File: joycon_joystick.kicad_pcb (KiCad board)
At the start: 2 copper layers, 35.1 x 23 mm, 2 parts, among them CN1 CONN_5POS, J1 Conn_01x05

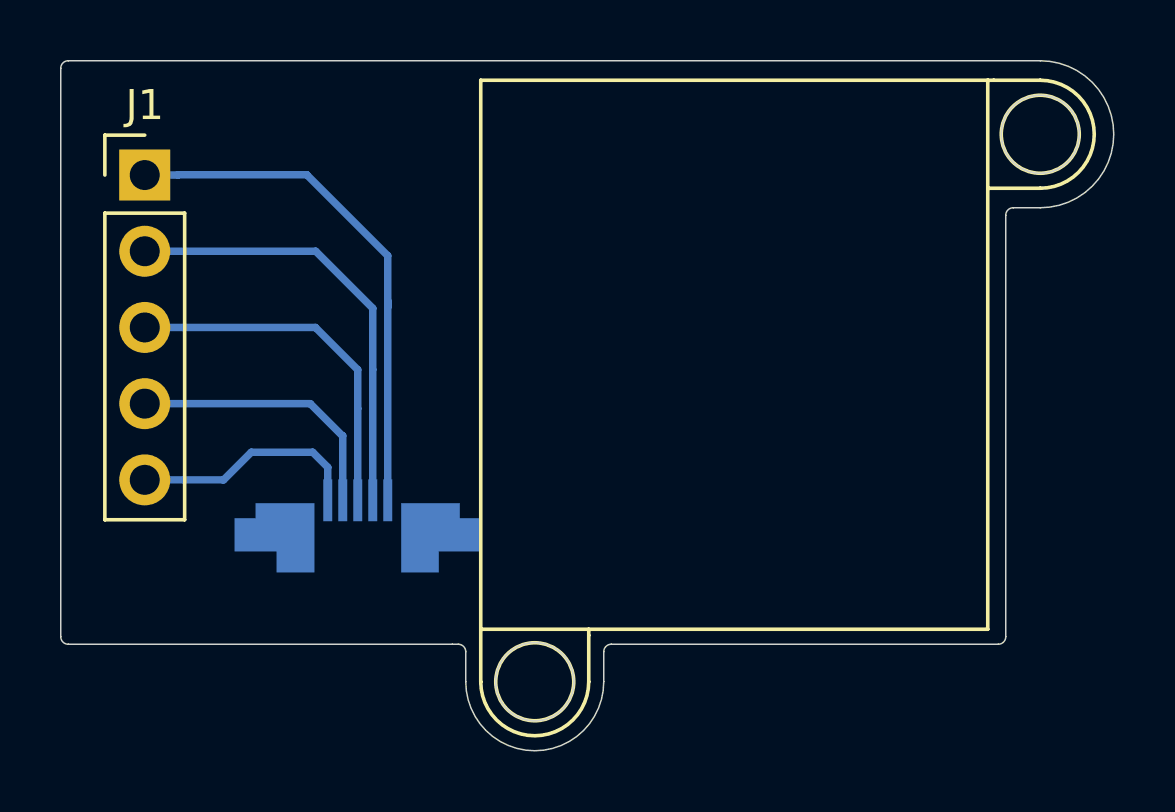
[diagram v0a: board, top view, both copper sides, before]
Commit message: took another shot at getting the geometry right
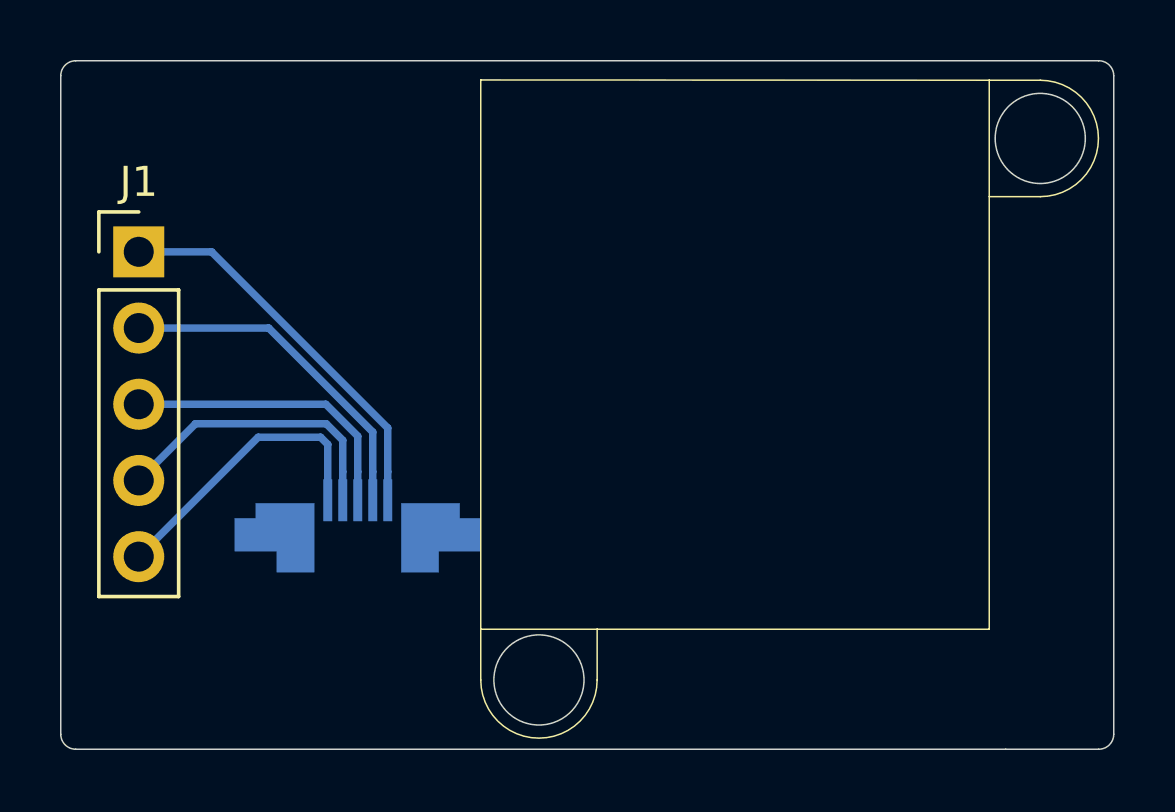
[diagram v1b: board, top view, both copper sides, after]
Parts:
- moved J1 2.57 mm to (117.6, 94.4)
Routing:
- net Net-(CN1-Pad1): track 17.6 -> 13.1 mm
- net Net-(CN1-Pad2): track 14.8 -> 11.5 mm
- net Net-(CN1-Pad3): track 12.0 -> 9.88 mm
- net Net-(CN1-Pad5): track 7.79 -> 9.91 mm
- net Net-(CN1-Pad4): track 9.19 -> 9.81 mm
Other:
- outline, holes or cut-outs redrawn
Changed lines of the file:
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@@
   (general
     (thickness 1.6)
-    (drawings 41)
-    (tracks 24)
+    (drawings 29)
+    (tracks 21)
     (zones 0)
     (modules 2)
@@
   )
   (module Connector_PinHeader_2.54mm:PinHeader_1x05_P2.54mm_Vertical (layer F.Cu)
-    (at 117.8 91.86)
+    (at 117.6 94.42)
     (descr "Through hole straight pin header, 1x05, 2.54mm pitch, single row")
     (tags "Through hole pin header THT 1x05 2.54mm single row")
@@
     )
   )
-  (gr_circle (center 130.8 108.75) (end 129.7 109.45) (layer Edge.Cuts) (width 0.05))
-  (gr_circle (center 147.65 90.5) (end 148.95 90.5) (layer Edge.Cuts) (width 0.05))
-  (gr_arc (start 146.75 93.2) (end 146.75 92.95) (angle -90) (layer Edge.Cuts) (width 0.05))
-  (gr_arc (start 146.25 107.25) (end 146.25 107.5) (angle -90) (layer Edge.Cuts) (width 0.05))
-  (gr_arc (start 133.35 107.75) (end 133.35 107.5) (angle -90) (layer Edge.Cuts) (width 0.05))
-  (gr_line (start 128.05 107.5) (end 128.25 107.5) (layer Edge.Cuts) (width 0.05))
-  (gr_arc (start 128.25 107.75) (end 128.5 107.75) (angle -90) (layer Edge.Cuts) (width 0.05))
-  (gr_line (start 115.25 107.5) (end 128.05 107.5) (layer Edge.Cuts) (width 0.05))
-  (gr_line (start 115 107.25) (end 115 88.3) (layer Edge.Cuts) (width 0.05))
-  (gr_arc (start 115.25 107.25) (end 115 107.25) (angle -90) (layer Edge.Cuts) (width 0.05))
-  (gr_line (start 115.25 88.05) (end 147.65 88.05) (layer Edge.Cuts) (width 0.05))
-  (gr_arc (start 115.25 88.3) (end 115.25 88.05) (angle -90) (layer Edge.Cuts) (width 0.05))
-  (gr_line (start 147.65 92.95) (end 146.75 92.95) (layer Edge.Cuts) (width 0.05))
-  (gr_line (start 133.35 107.5) (end 146.25 107.5) (layer Edge.Cuts) (width 0.05))
-  (gr_line (start 128.5 108.75) (end 128.5 107.75) (layer Edge.Cuts) (width 0.05))
-  (gr_line (start 133.1 108.75) (end 133.1 107.75) (layer Edge.Cuts) (width 0.05))
-  (gr_arc (start 130.8 108.75) (end 128.5 108.75) (angle -180) (layer Edge.Cuts) (width 0.05))
-  (gr_arc (start 147.65 90.5) (end 147.65 92.95) (angle -180) (layer Edge.Cuts) (width 0.05))
-  (gr_line (start 146.5 107.25) (end 146.5 93.2) (layer Edge.Cuts) (width 0.05))
+  (gr_arc (start 115.5 88.55) (end 115.5 88.05) (angle -90) (layer Edge.Cuts) (width 0.05))
+  (gr_arc (start 115.5 110.5) (end 115 110.5) (angle -90) (layer Edge.Cuts) (width 0.05))
+  (gr_arc (start 149.6 110.5) (end 149.6 111) (angle -90) (layer Edge.Cuts) (width 0.05))
+  (gr_arc (start 149.6 88.55) (end 150.1 88.55) (angle -90) (layer Edge.Cuts) (width 0.05))
+  (gr_line (start 132.88 106.99) (end 132.88 108.69) (layer F.SilkS) (width 0.05))
+  (gr_line (start 129 106.99) (end 129 108.69) (layer F.SilkS) (width 0.05))
+  (gr_circle (center 130.94 108.69) (end 131.43 110.11) (layer Edge.Cuts) (width 0.05))
+  (gr_arc (start 130.94 108.69) (end 129 108.69) (angle -180) (layer F.SilkS) (width 0.05))
+  (gr_arc (start 147.65 90.64) (end 147.65 92.58) (angle -180) (layer F.SilkS) (width 0.05))
+  (gr_line (start 145.95 88.7) (end 147.65 88.7) (layer F.SilkS) (width 0.05))
+  (gr_line (start 145.95 92.58) (end 147.65 92.58) (layer F.SilkS) (width 0.05))
+  (gr_line (start 145.95 88.7) (end 145.95 107) (layer F.SilkS) (width 0.05))
+  (gr_line (start 129 88.69) (end 145.95 88.7) (layer F.SilkS) (width 0.05))
+  (gr_circle (center 147.65 90.64) (end 149.07 90.15) (layer Edge.Cuts) (width 0.05))
+  (gr_line (start 149.6 111) (end 146.5 111) (layer Edge.Cuts) (width 0.05))
+  (gr_line (start 150.1 88.55) (end 150.1 110.5) (layer Edge.Cuts) (width 0.05))
+  (gr_line (start 115.5 111) (end 146.5 111) (layer Edge.Cuts) (width 0.05))
+  (gr_line (start 115 110.5) (end 115 88.55) (layer Edge.Cuts) (width 0.05))
+  (gr_line (start 115.5 88.05) (end 149.6 88.05) (layer Edge.Cuts) (width 0.05))
   (gr_text Y (at 134.05 93.6) (layer B.SilkS)
     (effects (font (size 2 2) (thickness 0.15)) (justify mirror))
@@
   (gr_line (start 132 89.5) (end 134 91.5) (layer B.SilkS) (width 0.12))
   (gr_line (start 132 94.5) (end 132 89.5) (layer B.SilkS) (width 0.12))
-  (gr_arc (start 130.8 108.75) (end 129 108.75) (angle -180) (layer F.SilkS) (width 0.12))
-  (gr_line (start 132.6 107) (end 132.6 107.2) (layer F.SilkS) (width 0.12))
-  (gr_line (start 129 108.75) (end 129 107) (layer F.SilkS) (width 0.12))
-  (gr_line (start 132.6 107.2) (end 132.6 108.75) (layer F.SilkS) (width 0.12))
-  (gr_circle (center 130.8 108.75) (end 130.8 110.05) (layer F.SilkS) (width 0.12))
-  (gr_arc (start 147.65 90.5) (end 147.65 92.3) (angle -180) (layer F.SilkS) (width 0.12))
-  (gr_line (start 147.65 92.3) (end 145.9 92.3) (layer F.SilkS) (width 0.12))
-  (gr_line (start 146.1 88.7) (end 147.65 88.7) (layer F.SilkS) (width 0.12))
-  (gr_circle (center 147.65 90.5) (end 148.95 90.5) (layer F.SilkS) (width 0.12))
-  (gr_line (start 145.9 88.7) (end 146.1 88.7) (layer F.SilkS) (width 0.12))
-  (gr_line (start 129 88.7) (end 129 107) (layer F.SilkS) (width 0.12))
-  (gr_line (start 145.9 88.7) (end 129 88.7) (layer F.SilkS) (width 0.12))
-  (gr_line (start 145.9 107) (end 145.9 88.7) (layer F.SilkS) (width 0.12))
-  (gr_line (start 129 107) (end 145.9 107) (layer F.SilkS) (width 0.12))
-  (segment (start 118.9 91.86) (end 118.91 91.85) (width 0.25) (layer B.Cu) (net 1))
-  (segment (start 117.8 91.86) (end 118.9 91.86) (width 0.25) (layer B.Cu) (net 1))
-  (segment (start 118.91 91.85) (end 123.2 91.85) (width 0.25) (layer B.Cu) (net 1))
-  (segment (start 123.2 91.85) (end 125.9 94.55) (width 0.25) (layer B.Cu) (net 1))
-  (segment (start 125.9 96.25) (end 125.9 96.05) (width 0.25) (layer B.Cu) (net 1))
-  (segment (start 125.9 94.55) (end 125.9 96.25) (width 0.25) (layer B.Cu) (net 1))
-  (segment (start 125.9 102.7) (end 125.9 96.25) (width 0.25) (layer B.Cu) (net 1))
-  (segment (start 125.4 98.35) (end 125.4 102.7) (width 0.25) (layer B.Cu) (net 2))
-  (segment (start 117.8 94.4) (end 123.5 94.4) (width 0.25) (layer B.Cu) (net 2))
-  (segment (start 125.4 96.3) (end 125.4 98.35) (width 0.25) (layer B.Cu) (net 2))
-  (segment (start 123.5 94.4) (end 125.4 96.3) (width 0.25) (layer B.Cu) (net 2))
-  (segment (start 117.8 102.02) (end 120.43 102.02) (width 0.25) (layer B.Cu) (net 3))
-  (segment (start 120.43 102.02) (end 121.35 101.1) (width 0.25) (layer B.Cu) (net 3))
-  (segment (start 123.4 101.1) (end 123.9 101.6) (width 0.25) (layer B.Cu) (net 3))
-  (segment (start 121.35 101.1) (end 123.4 101.1) (width 0.25) (layer B.Cu) (net 3))
-  (segment (start 123.9 101.6) (end 123.9 102.7) (width 0.25) (layer B.Cu) (net 3))
-  (segment (start 124.4 100.55) (end 124.4 102.7) (width 0.25) (layer B.Cu) (net 4))
-  (segment (start 124.38641 100.55) (end 124.4 100.55) (width 0.25) (layer B.Cu) (net 4))
-  (segment (start 123.31641 99.48) (end 124.38641 100.55) (width 0.25) (layer B.Cu) (net 4))
-  (segment (start 117.8 99.48) (end 123.31641 99.48) (width 0.25) (layer B.Cu) (net 4))
-  (segment (start 124.9 99.65) (end 124.9 102.7) (width 0.25) (layer B.Cu) (net 5))
-  (segment (start 117.8 96.94) (end 123.49 96.94) (width 0.25) (layer B.Cu) (net 5))
-  (segment (start 124.9 98.35) (end 124.9 99.65) (width 0.25) (layer B.Cu) (net 5))
-  (segment (start 123.49 96.94) (end 124.9 98.35) (width 0.25) (layer B.Cu) (net 5))
+  (gr_line (start 129 88.69) (end 129 107) (layer F.SilkS) (width 0.05))
+  (gr_line (start 129 107) (end 145.95 107) (layer F.SilkS) (width 0.05))
+  (segment (start 125.9 101.75) (end 125.9 102.7) (width 0.25) (layer B.Cu) (net 1))
+  (segment (start 125.9 100.29077) (end 125.9 101.75) (width 0.25) (layer B.Cu) (net 1))
+  (segment (start 120.02923 94.42) (end 125.9 100.29077) (width 0.25) (layer B.Cu) (net 1))
+  (segment (start 117.6 94.42) (end 120.02923 94.42) (width 0.25) (layer B.Cu) (net 1))
+  (segment (start 125.4 100.42718) (end 125.4 101.75) (width 0.25) (layer B.Cu) (net 2))
+  (segment (start 121.93282 96.96) (end 125.4 100.42718) (width 0.25) (layer B.Cu) (net 2))
+  (segment (start 125.4 101.75) (end 125.4 102.7) (width 0.25) (layer B.Cu) (net 2))
+  (segment (start 117.6 96.96) (end 121.93282 96.96) (width 0.25) (layer B.Cu) (net 2))
+  (segment (start 117.6 104.58) (end 121.58 100.6) (width 0.25) (layer B.Cu) (net 3))
+  (segment (start 121.58 100.6) (end 123.66359 100.6) (width 0.25) (layer B.Cu) (net 3))
+  (segment (start 123.9 100.83641) (end 123.9 102.7) (width 0.25) (layer B.Cu) (net 3))
+  (segment (start 123.66359 100.6) (end 123.9 100.83641) (width 0.25) (layer B.Cu) (net 3))
+  (segment (start 124.4 101.75) (end 124.4 102.7) (width 0.25) (layer B.Cu) (net 4))
+  (segment (start 124.4 100.7) (end 124.4 101.75) (width 0.25) (layer B.Cu) (net 4))
+  (segment (start 123.85 100.15) (end 124.4 100.7) (width 0.25) (layer B.Cu) (net 4))
+  (segment (start 119.49 100.15) (end 123.85 100.15) (width 0.25) (layer B.Cu) (net 4))
+  (segment (start 117.6 102.04) (end 119.49 100.15) (width 0.25) (layer B.Cu) (net 4))
+  (segment (start 124.9 101.75) (end 124.9 102.7) (width 0.25) (layer B.Cu) (net 5))
+  (segment (start 124.9 100.56359) (end 124.9 101.75) (width 0.25) (layer B.Cu) (net 5))
+  (segment (start 123.83641 99.5) (end 124.9 100.56359) (width 0.25) (layer B.Cu) (net 5))
+  (segment (start 117.6 99.5) (end 123.83641 99.5) (width 0.25) (layer B.Cu) (net 5))
 )
